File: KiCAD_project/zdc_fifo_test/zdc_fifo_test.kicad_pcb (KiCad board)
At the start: 2 copper layers, 0 parts

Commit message: Started PCB layout
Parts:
- added C1: 0.1n, Capacitor_SMD:C_0402_1005Metric, F.Cu at (213.6, 96.8)
- added C10: 0.1n, Capacitor_SMD:C_0402_1005Metric, F.Cu at (213.6, 108.6)
- added C11: 10u, Capacitor_SMD:C_0805_2012Metric, F.Cu at (166.9, 107.5)
- added C12: 1n, Capacitor_SMD:C_0402_1005Metric, F.Cu at (213.6, 110.6)
- added C13: 0.1n, Capacitor_SMD:C_0402_1005Metric, F.Cu at (213.6, 112.5)
- added C2: 1n, Capacitor_SMD:C_0402_1005Metric, F.Cu at (213.6, 98.7)
- added C20: 100u, Library_footprints:CAP-SMD_BD6.3-L6.6-W6.6-LS7.6-FD-1, F.Cu at (180.0, 157.0)
- added C21: 1n, Capacitor_SMD:C_0402_1005Metric, F.Cu at (216.4, 96.8)
- added C22: 0.1n, Capacitor_SMD:C_0402_1005Metric, F.Cu at (216.4, 98.7)
- added C23: 10u, Capacitor_SMD:C_0805_2012Metric, F.Cu at (166.9, 110.5)
- added C24: 1n, Capacitor_SMD:C_0402_1005Metric, F.Cu at (216.4, 100.7)
- added C25: 0.1n, Capacitor_SMD:C_0402_1005Metric, F.Cu at (216.4, 102.7)
- added C26: 100n, Capacitor_SMD:C_0402_1005Metric, F.Cu at (216.4, 104.7)
- added C27: 1u, Capacitor_SMD:C_0603_1608Metric, F.Cu at (192.2, 106.0)
- added C28: 1n, Capacitor_SMD:C_0402_1005Metric, F.Cu at (216.4, 106.6)
- added C29: 100n, Capacitor_SMD:C_0402_1005Metric, F.Cu at (216.4, 108.6)
- added C3: 100u, Library_footprints:CAP-SMD_BD6.3-L6.6-W6.6-LS7.6-FD-1, F.Cu at (206.5, 185.5)
- added C30: 1u, Capacitor_SMD:C_0603_1608Metric, F.Cu at (192.2, 108.5)
- added C31: 100u, Library_footprints:CAP-SMD_BD6.3-L6.6-W6.6-LS7.6-FD-1, F.Cu at (194.0, 157.5)
- added C32: 1n, Capacitor_SMD:C_0402_1005Metric, F.Cu at (216.4, 110.6)
- added C33: 0.1n, Capacitor_SMD:C_0402_1005Metric, F.Cu at (216.4, 112.5)
- added C34: 10u, Capacitor_SMD:C_0805_2012Metric, F.Cu at (166.9, 113.5)
- added C35: 1n, Capacitor_SMD:C_0402_1005Metric, F.Cu at (219.3, 96.8)
- added C36: 0.1n, Capacitor_SMD:C_0402_1005Metric, F.Cu at (219.3, 98.7)
- added C4: 1n, Capacitor_SMD:C_0402_1005Metric, F.Cu at (213.6, 100.7)
- added C5: 10u, Capacitor_SMD:C_0805_2012Metric, F.Cu at (166.9, 104.5)
- added C55: 1n, Capacitor_SMD:C_0402_1005Metric, F.Cu at (219.3, 100.7)
- added C56: 100n, Capacitor_SMD:C_0402_1005Metric, F.Cu at (219.3, 102.7)
- added C57: 1u, Capacitor_SMD:C_0603_1608Metric, F.Cu at (192.2, 111.0)
- added C58: 1n, Capacitor_SMD:C_0402_1005Metric, F.Cu at (219.3, 104.7)
- added C59: 100n, Capacitor_SMD:C_0402_1005Metric, F.Cu at (219.3, 106.6)
- added C6: 1n, Capacitor_SMD:C_0402_1005Metric, F.Cu at (213.6, 102.7)
- added C60: 1u, Capacitor_SMD:C_0603_1608Metric, F.Cu at (192.2, 113.5)
- added C61: 1u, Capacitor_SMD:C_0603_1608Metric, F.Cu at (192.2, 116.0)
- added C62: 100n, Capacitor_SMD:C_0402_1005Metric, F.Cu at (219.3, 108.6)
- added C63: 1n, Capacitor_SMD:C_0402_1005Metric, F.Cu at (219.3, 110.6)
- added C64: 1n, Capacitor_SMD:C_0402_1005Metric, F.Cu at (219.3, 112.5)
- added C65: 100n, Capacitor_SMD:C_0402_1005Metric, F.Cu at (222.2, 96.8)
- added C66: 1u, Capacitor_SMD:C_0603_1608Metric, F.Cu at (196.2, 106.0)
- added C67: 1u, Capacitor_SMD:C_0603_1608Metric, F.Cu at (196.2, 108.5)
- added C68: 100n, Capacitor_SMD:C_0402_1005Metric, F.Cu at (222.2, 98.7)
- added C69: 1n, Capacitor_SMD:C_0402_1005Metric, F.Cu at (222.2, 100.7)
- added C7: 0.1n, Capacitor_SMD:C_0402_1005Metric, F.Cu at (213.6, 104.7)
- added C70: 1n, Capacitor_SMD:C_0402_1005Metric, F.Cu at (222.2, 102.7)
- added C71: 100n, Capacitor_SMD:C_0402_1005Metric, F.Cu at (222.2, 104.7)
- added C72: 1u, Capacitor_SMD:C_0603_1608Metric, F.Cu at (196.2, 111.0)
- added C73: 1u, Capacitor_SMD:C_0603_1608Metric, F.Cu at (196.2, 113.5)
- added C74: 100n, Capacitor_SMD:C_0402_1005Metric, F.Cu at (222.2, 106.6)
- added C75: 1n, Capacitor_SMD:C_0402_1005Metric, F.Cu at (222.2, 108.6)
- added C76: 1n, Capacitor_SMD:C_0402_1005Metric, F.Cu at (222.2, 110.6)
- added C77: 100n, Capacitor_SMD:C_0402_1005Metric, F.Cu at (222.2, 112.5)
- added C78: 1u, Capacitor_SMD:C_0603_1608Metric, F.Cu at (196.2, 116.0)
- added C8: 100u, Library_footprints:CAP-SMD_BD6.3-L6.6-W6.6-LS7.6-FD-1, F.Cu at (219.8, 185.5)
- added C9: 1n, Capacitor_SMD:C_0402_1005Metric, F.Cu at (213.6, 106.6)
- added IC1: OPA695IDR, Library_footprints:SOIC127P600X175-8N, F.Cu at (173.2, 78.1)
- added IC2: AD8009ARZ, Library_footprints:SOIC127P600X175-8N, F.Cu at (243.1, 70.7)
- added IC3: AD8009ARZ, Library_footprints:SOIC127P600X175-8N, F.Cu at (232.5, 70.5)
- added IC4: AD8009ARZ, Library_footprints:SOIC127P600X175-8N, F.Cu at (220.5, 70.5)
- added IC5: AD8009ARZ, Library_footprints:SOIC127P600X175-8N, F.Cu at (210.0, 70.5)
- added IC6: L7905ACD2T-TR, Library_footprints:STB20N95K5, F.Cu at (180.1, 170.9)
- added IC7: L7905ACD2T-TR, Library_footprints:STB20N95K5, F.Cu at (193.3, 170.9)
- added IC8: L7805ACD2T-TR, Library_footprints:L7805ACD2TTR, F.Cu at (206.5, 170.9)
- added IC9: L7805ACD2T-TR, Library_footprints:L7805ACD2TTR, F.Cu at (219.7, 170.9)
- added J1: EPL.00.250.NTN, Library_footprints:CONN_EPK.00.250.NTN_LMO, F.Cu at (156.6, 59.5)
- added J2: EPL.00.250.NTN, Library_footprints:CONN_EPK.00.250.NTN_LMO, F.Cu at (167.7, 59.5)
- added J3: EPL.00.250.NTN, Library_footprints:CONN_EPK.00.250.NTN_LMO, F.Cu at (178.9, 59.5)
- added J4: EPL.00.250.NTN, Library_footprints:CONN_EPK.00.250.NTN_LMO, F.Cu at (190.0, 59.5)
- added J5: EPL.00.250.NTN, Library_footprints:CONN_EPK.00.250.NTN_LMO, F.Cu at (210.4, 59.5)
- added J6: EPL.00.250.NTN, Library_footprints:CONN_EPK.00.250.NTN_LMO, F.Cu at (221.5, 59.5)
- added J7: EPL.00.250.NTN, Library_footprints:CONN_EPK.00.250.NTN_LMO, F.Cu at (232.6, 59.5)
- added J8: EPL.00.250.NTN, Library_footprints:CONN_EPK.00.250.NTN_LMO, F.Cu at (243.8, 59.5)
- added R17: 123, Resistor_SMD:R_0402_1005Metric, F.Cu at (194.7, 79.5)
- added R18: 402, Resistor_SMD:R_0402_1005Metric, F.Cu at (194.7, 84.0)
- added R19: 134, Resistor_SMD:R_0402_1005Metric, F.Cu at (194.7, 86.0)
- added R20: 50, Resistor_SMD:R_0402_1005Metric, F.Cu at (194.7, 88.0)
- added R21: 50, Resistor_SMD:R_0402_1005Metric, F.Cu at (194.7, 90.0)
- added R22: 50, Resistor_SMD:R_0402_1005Metric, F.Cu at (194.7, 92.0)
- added R23: 50, Resistor_SMD:R_0402_1005Metric, F.Cu at (194.7, 94.0)
- added R24: 50, Resistor_SMD:R_0402_1005Metric, F.Cu at (197.6, 79.5)
- added R25: 50, Resistor_SMD:R_0402_1005Metric, F.Cu at (197.6, 84.0)
- added R26: 50, Resistor_SMD:R_0402_1005Metric, F.Cu at (197.6, 86.0)
- added R27: 50, Resistor_SMD:R_0402_1005Metric, F.Cu at (197.6, 88.0)
- added R28: 51, Resistor_SMD:R_0402_1005Metric, F.Cu at (244.0, 64.5)
- added R29: 250, Resistor_SMD:R_0402_1005Metric, F.Cu at (197.6, 92.0)
- added R30: 250, Resistor_SMD:R_0402_1005Metric, F.Cu at (197.6, 94.0)
- added R31: 2k, Resistor_SMD:R_0402_1005Metric, F.Cu at (200.5, 79.5)
- added R32: 2k, Resistor_SMD:R_0402_1005Metric, F.Cu at (200.5, 84.0)
- added R33: 250, Resistor_SMD:R_0402_1005Metric, F.Cu at (200.5, 86.0)
- added R34: 250, Resistor_SMD:R_0402_1005Metric, F.Cu at (200.5, 88.0)
- added R35: 51, Resistor_SMD:R_0402_1005Metric, F.Cu at (233.0, 64.5)
- added R36: 2k, Resistor_SMD:R_0402_1005Metric, F.Cu at (200.5, 92.0)
- added R37: 250, Resistor_SMD:R_0402_1005Metric, F.Cu at (200.5, 94.0)
- added R38: 250, Resistor_SMD:R_0402_1005Metric, F.Cu at (210.0, 88.5)
- added R39: 51, Resistor_SMD:R_0402_1005Metric, F.Cu at (221.5, 64.5)
- added R40: 2k, Resistor_SMD:R_0402_1005Metric, F.Cu at (203.4, 86.0)
- added R41: 250, Resistor_SMD:R_0402_1005Metric, F.Cu at (203.4, 88.0)
- added R42: 250, Resistor_SMD:R_0402_1005Metric, F.Cu at (203.4, 90.0)
- added R43: 51, Resistor_SMD:R_0402_1005Metric, F.Cu at (210.5, 64.5)
- added U1: ~, Library_footprints:CONN-TH_XY126V-5.0-3P, F.Cu at (202.5, 195.0)
- added VR2: 3006P-1-502LF, Library_footprints:3006P_1, F.Cu at (202.4, 69.7)
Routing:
- added copper zone on In2.Cu, net +5V_stg1
- added copper zone on In2.Cu, net +5V_stg2
- added copper zone on In3.Cu, net -5V_stg1
- added copper zone on In3.Cu, net -5V_stg2
- added copper zone on In1.Cu, net GND
- added copper zone on In4.Cu, net GND
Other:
- board outline added: 100 x 150 mm
- copper layers 2 -> 6
- board text added: "INPUT"

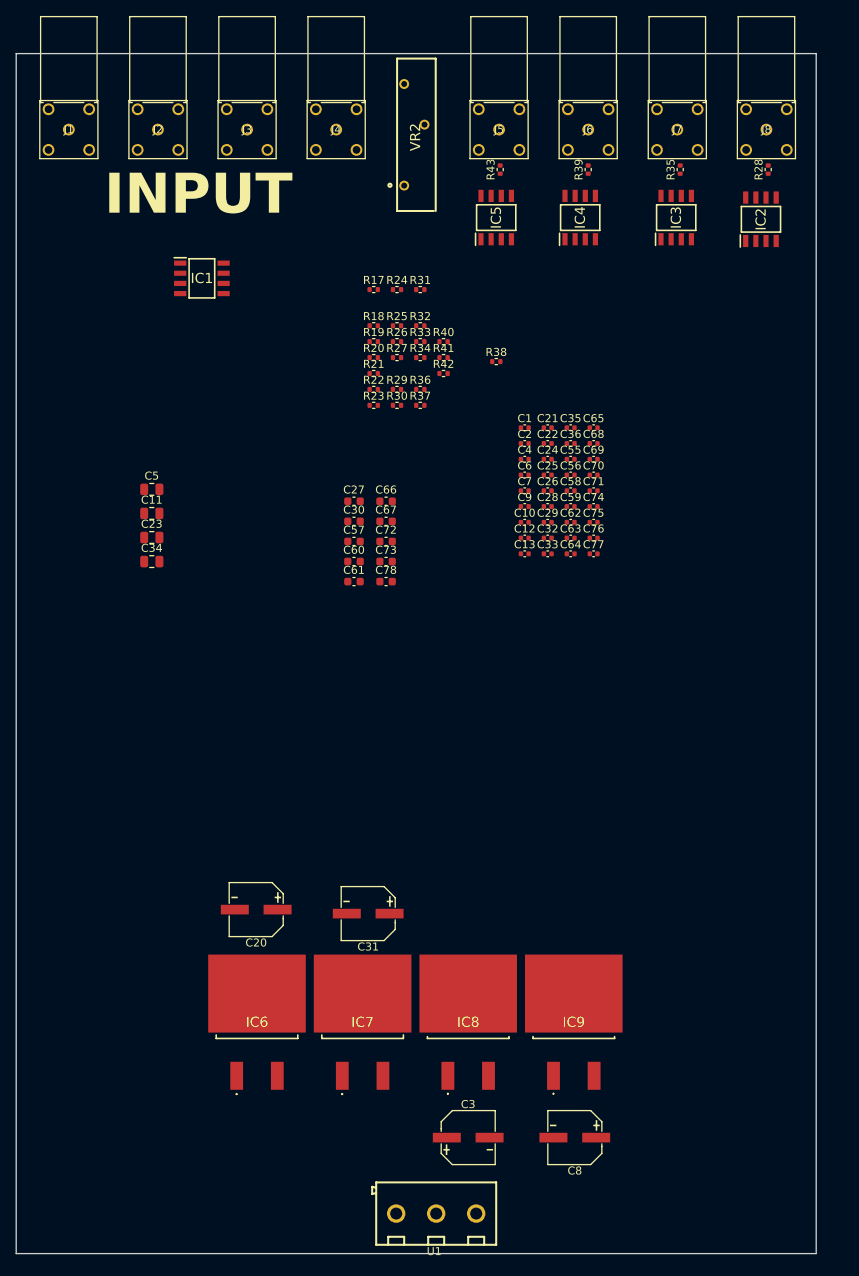
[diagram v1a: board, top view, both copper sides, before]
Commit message: first gerber generated
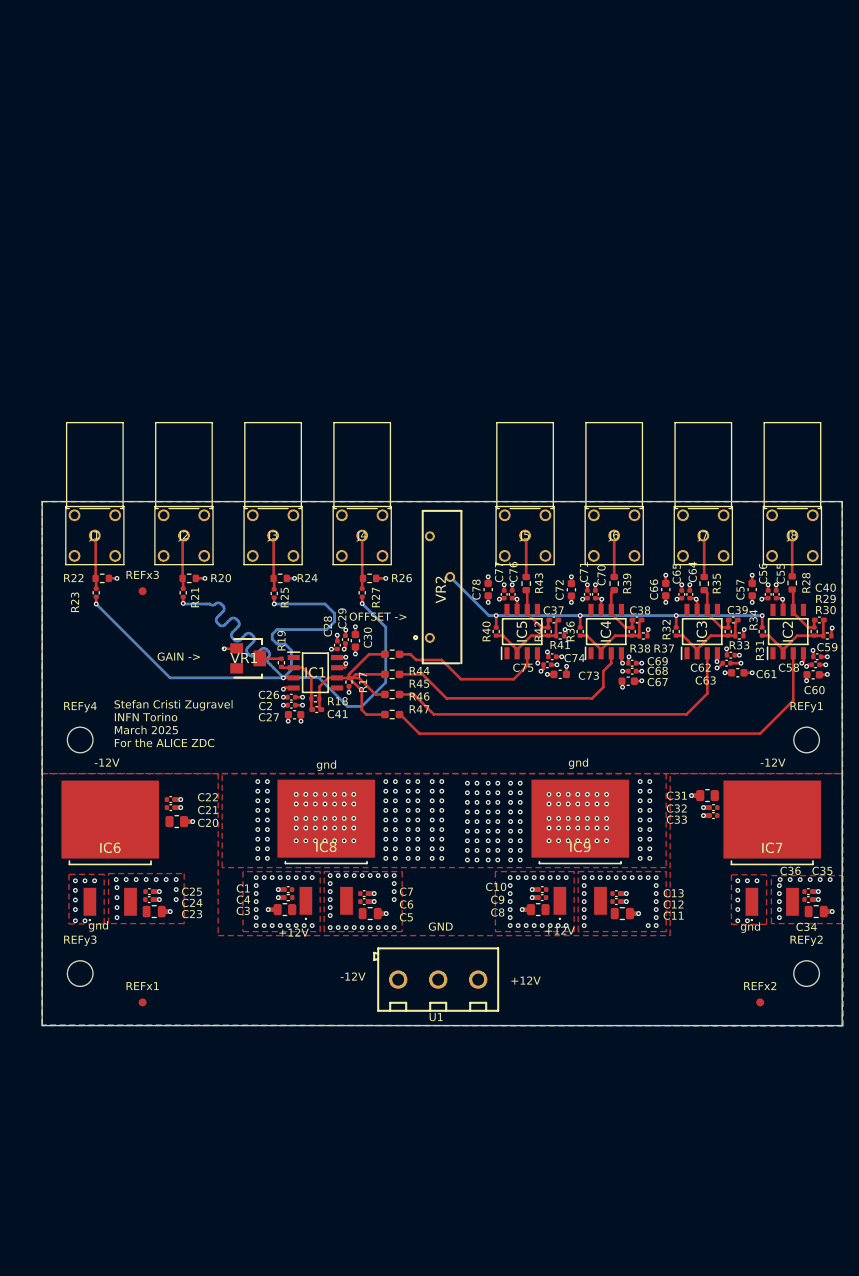
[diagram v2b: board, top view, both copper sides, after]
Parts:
- added C37: NM, Capacitor_SMD:C_0402_1005Metric_Pad0.74x0.62mm_HandSolder, F.Cu at (217.2, 120.8)
- added C38: NM, Capacitor_SMD:C_0402_1005Metric_Pad0.74x0.62mm_HandSolder, F.Cu at (227.6, 120.8)
- added C39: NM, Capacitor_SMD:C_0402_1005Metric_Pad0.74x0.62mm_HandSolder, F.Cu at (239.6, 120.8)
- added C40: NM, Capacitor_SMD:C_0402_1005Metric_Pad0.74x0.62mm_HandSolder, F.Cu at (250.4, 120.8)
- added C41: NM, Capacitor_SMD:C_0402_1005Metric_Pad0.74x0.62mm_HandSolder, F.Cu at (187.6, 132.0)
- added R44: 0, Resistor_SMD:R_0603_1608Metric_Pad0.98x0.95mm_HandSolder, F.Cu at (197.0, 125.1)
- added R45: 0, Resistor_SMD:R_0603_1608Metric_Pad0.98x0.95mm_HandSolder, F.Cu at (197.0, 127.6)
- added R46: 0, Resistor_SMD:R_0603_1608Metric_Pad0.98x0.95mm_HandSolder, F.Cu at (197.0, 130.1)
- added R47: 0, Resistor_SMD:R_0603_1608Metric_Pad0.98x0.95mm_HandSolder, F.Cu at (197.0, 132.6)
- added REFx1: Fiducial_1mm_Mask2mm, Fiducial:Fiducial_1mm_Mask2mm, F.Cu at (165.8, 168.6)
- added REFx2: Fiducial_1mm_Mask2mm, Fiducial:Fiducial_1mm_Mask2mm, F.Cu at (243.0, 168.6)
- added REFx3: Fiducial_1mm_Mask2mm, Fiducial:Fiducial_1mm_Mask2mm, F.Cu at (165.8, 117.2)
- added REFy1: MountingHole_3.2mm_M3, MountingHole:MountingHole_3.2mm_M3, F.Cu at (248.8, 135.8)
- added REFy2: MountingHole_3.2mm_M3, MountingHole:MountingHole_3.2mm_M3, F.Cu at (248.8, 165.0)
- added REFy3: MountingHole_3.2mm_M3, MountingHole:MountingHole_3.2mm_M3, F.Cu at (158.0, 165.0)
- added REFy4: MountingHole_3.2mm_M3, MountingHole:MountingHole_3.2mm_M3, F.Cu at (158.0, 135.8)
- added VR1: 3224W-1-500E, Library_footprints:3224W1500E, F.Cu at (179.0, 125.6)
- C1, C10, C22, C33: value 0.1n -> 100n
- C12, C24, C35, C6: value 1n -> 100n
- C13, C25, C36, C7: value 0.1n -> 1n
- C20, C3, C31, C8: value 100u -> 10u; footprint Library_footprints:CAP-SMD_BD6.3-L6.6-W6.6-LS7.6-FD-1 -> Resistor_SMD:R_0805_2012Metric
- C21, C32, C9: value 1n -> 1u
- C4: value 1n -> 1u; footprint Capacitor_SMD:C_0402_1005Metric -> Resistor_SMD:R_0402_1005Metric
- R19: value 134 -> 100
- R20, R22, R24, R26, R28, R35, R39, R43: footprint Resistor_SMD:R_0402_1005Metric -> Resistor_SMD:R_0603_1608Metric
- moved C34 93.9 mm to (250.0, 157.2), turned to 180 degrees
- moved C11 77.2 mm to (225.8, 157.5)
- moved C24 74.2 mm to (166.6, 155.8), turned to 180 degrees
- moved C25 72.0 mm to (166.6, 154.8), turned to 180 degrees
- moved C21 66.9 mm to (169.3, 144.2), turned to 180 degrees
- moved C35 66.0 mm to (249.0, 155.8), turned to 180 degrees
- moved C1 64.9 mm to (184.0, 154.5), turned to 180 degrees
- moved C22 64.8 mm to (169.3, 143.2), turned to 180 degrees
- moved C36 63.4 mm to (249.0, 154.8), turned to 180 degrees
- moved C4 62.3 mm to (184.0, 155.5), turned to 180 degrees
- moved R30 61.0 mm to (251.4, 122.8), turned to 180 degrees
- moved R31 60.5 mm to (243.2, 122.2), turned to 90 degrees
- moved R29 60.3 mm to (249.8, 122.2), turned to 90 degrees
- moved C5 59.6 mm to (194.2, 157.5)
- moved C60 59.1 mm to (249.6, 127.7)
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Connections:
- IC2 pad 3: Net-(IC1-OUTPUT) -> Net-(IC2-+IN)
- IC3 pad 3: Net-(IC1-OUTPUT) -> Net-(IC3-+IN)
- IC4 pad 3: Net-(IC1-OUTPUT) -> Net-(IC4-+IN)
- IC5 pad 3: Net-(IC1-OUTPUT) -> Net-(IC5-+IN)
- R19 pad 1: GND -> Net-(VR1-WIPER)
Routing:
- net Net-(IC1-NONINVERTING_INPUT): track 0.00 -> 110.1 mm, vias 0 -> 5
- net GND: track 0.00 -> 60.8 mm, vias 0 -> 294
- net Net-(IC2-+IN): track 0.00 -> 57.8 mm
- net Net-(VR2-WIPER): track 0.00 -> 47.0 mm, vias 0 -> 4
- net Net-(IC3-+IN): track 0.00 -> 45.6 mm
- net Net-(IC4-+IN): track 0.00 -> 32.0 mm
- net Net-(IC1-OUTPUT): track 0.00 -> 30.5 mm
- net Net-(IC5-+IN): track 0.00 -> 19.5 mm
- net +5V_stg2: track 0.00 -> 15.5 mm, vias 0 -> 35
- net -5V_stg2: track 0.00 -> 15.0 mm, vias 0 -> 27
- net Net-(IC5--IN): track 0.00 -> 12.1 mm
- net Net-(IC3--IN): track 0.00 -> 11.9 mm
- net Net-(IC2--IN): track 0.00 -> 11.6 mm
- net Net-(IC4--IN): track 0.00 -> 11.4 mm
- net Net-(IC1-INVERTING_INPUT): track 0.00 -> 8.42 mm
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- added copper zone on F.Cu, net +12V_NIM
- added copper zone on In4.Cu, net +12V_NIM
- added copper zone on F.Cu, net +5V_stg1
- added copper zone on F.Cu, net +5V_stg2
- added copper zone on F.Cu, net -12V_NIM
- added copper zone on F.Cu, net -5V_stg1
- added copper zone on F.Cu, net -5V_stg2
- added copper zone on B.Cu, net GND
- added copper zone on F.Cu, net GND
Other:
- board size 100 x 150 mm -> 100 x 65.5 mm
- board text added: "+12V"
- board text added: "-12V"
- board text added: "GAIN ->"
- board text added: "GND"
- board text added: "OFFSET ->"
- board text added: "Stefan Cristi Zugravel INFN Torino March 2025 For the ALICE ZDC"
- board text added: "gnd"
- board text removed: "INPUT"
